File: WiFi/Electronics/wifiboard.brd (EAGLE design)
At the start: 94.9 x 41.9 mm, 16 parts, among them IC2 7805DT, Q2 IPB45N04, X1 MKDSN1,5/2-5,08, X2 MKDSN1,5/2-5,08

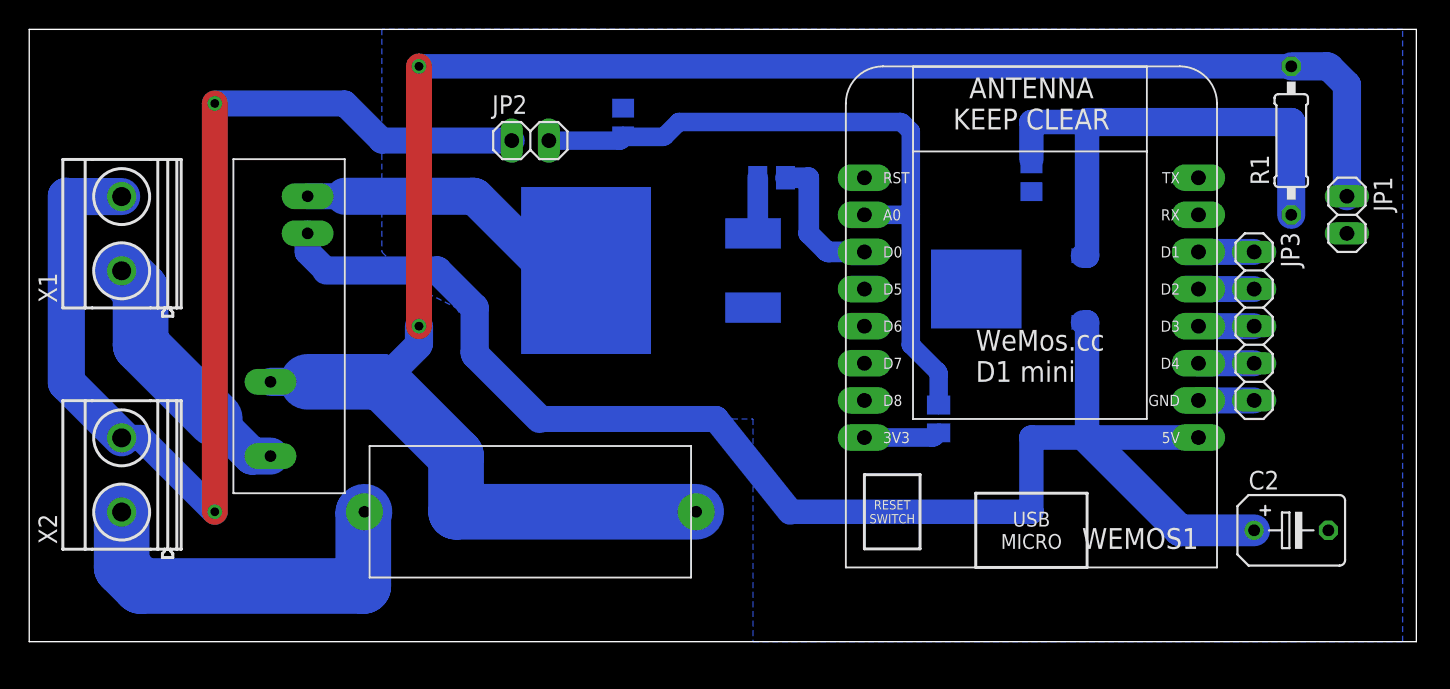
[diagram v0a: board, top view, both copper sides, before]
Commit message: Improved PCB design and casing.
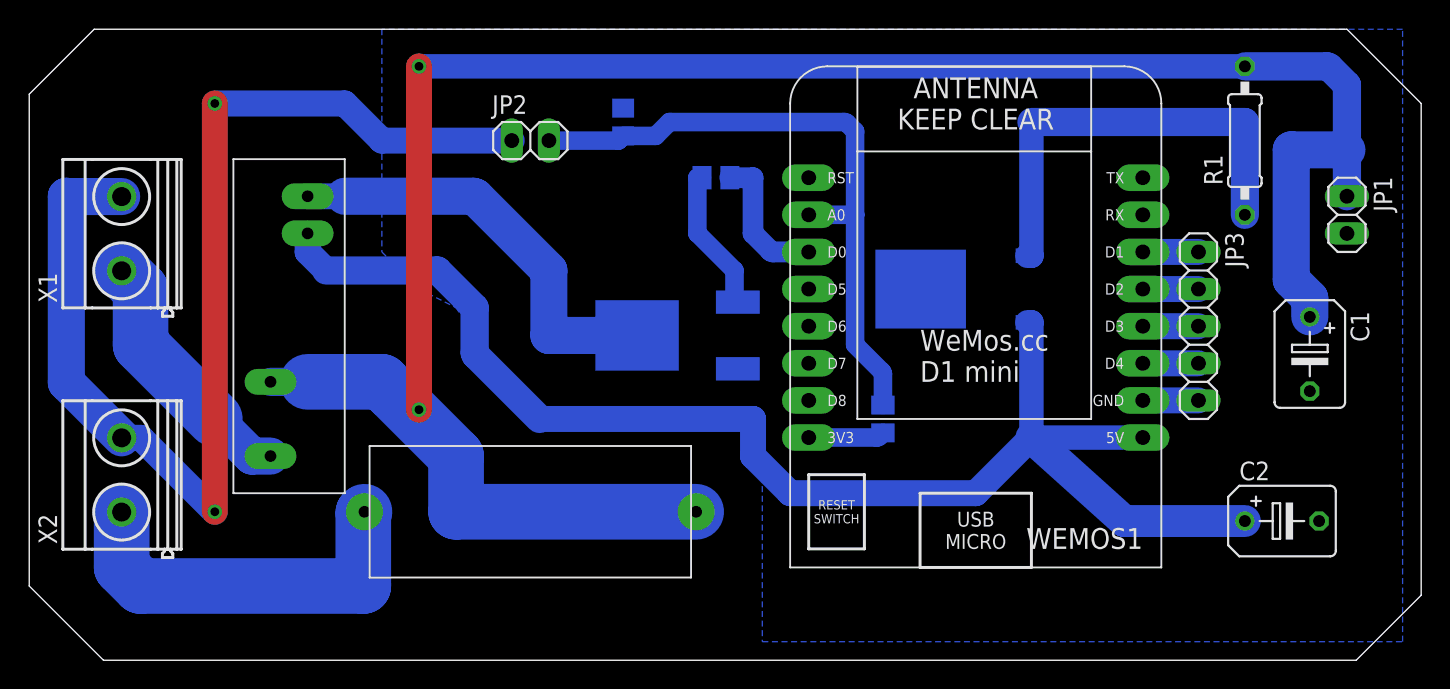
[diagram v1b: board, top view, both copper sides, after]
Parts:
- removed Q2: IPB45N04, transistor-power:D2PACK
- added Q1: FDD8870, SparkFun-DiscreteSemi:DPAK
- C1: value 47uF -> 1000uF; device rcl:C0805 -> rcl:B45181B
- moved C1 22.5 mm to (87.6, 19.7), flipped to the top
- moved IC2 3.81 mm to (63.5, 24.1)
- moved WEMOS1 3.81 mm to (63.5, 24.1)
- moved R2 3.81 mm to (58.4, 15.2)
- moved R3 3.81 mm to (47.0, 31.8)
- moved JP3 3.81 mm to (80.0, 21.6)
- moved R1 3.17 mm to (83.2, 34.3)
- moved C2 0.90 mm to (85.7, 8.26)
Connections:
- net +12V: now also C1.+
- net GND: now also C1.-, Q1.3; no longer C1.2, Q2.3
- net N$2: no longer C1.1
- net N$5: now also Q1.1; no longer Q2.1
- net N$7: now also Q1.4; no longer Q2.2
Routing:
- net +12V: track 129.3 -> 148.4 mm
- net N$7: track 21.1 -> 29.1 mm
- net N$5: track 3.93 -> 9.98 mm
- net N$2: track 36.4 -> 30.4 mm
- net +5V: track 99.2 -> 95.1 mm
- net N$3: track 48.3 -> 44.4 mm
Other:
- board size 94.9 x 41.9 mm -> 95.2 x 43.2 mm
